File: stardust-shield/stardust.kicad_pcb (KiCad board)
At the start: 2 copper layers, 112.4 x 85.5 mm, 64 parts, among them J1 BEXUS 28V, J2 Pololu J8557, J3 Pololu J8557, J4 Pololu J9251, J5 Pololu J9251 Servo, J6 DS3231M, J7 VMA430, J7'1 VMA430, SW1 SW_Push, SW2 SW_Push, U1 INA181, U2 INA181, U3 INA181, U4 INA181, U5 DS18B20, U6 DS18B20, U8 DHT22, U9 SSCDRNN015PASA5

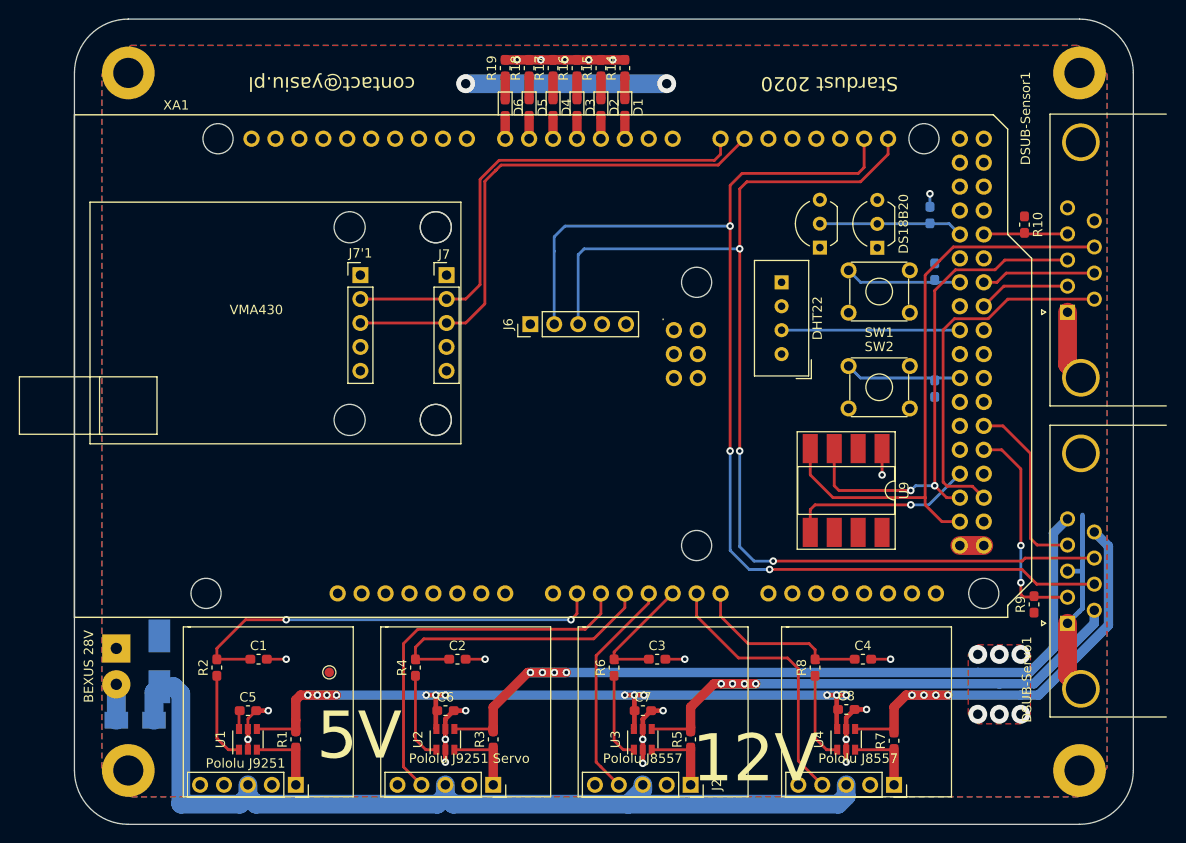
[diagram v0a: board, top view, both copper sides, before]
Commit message: change everything
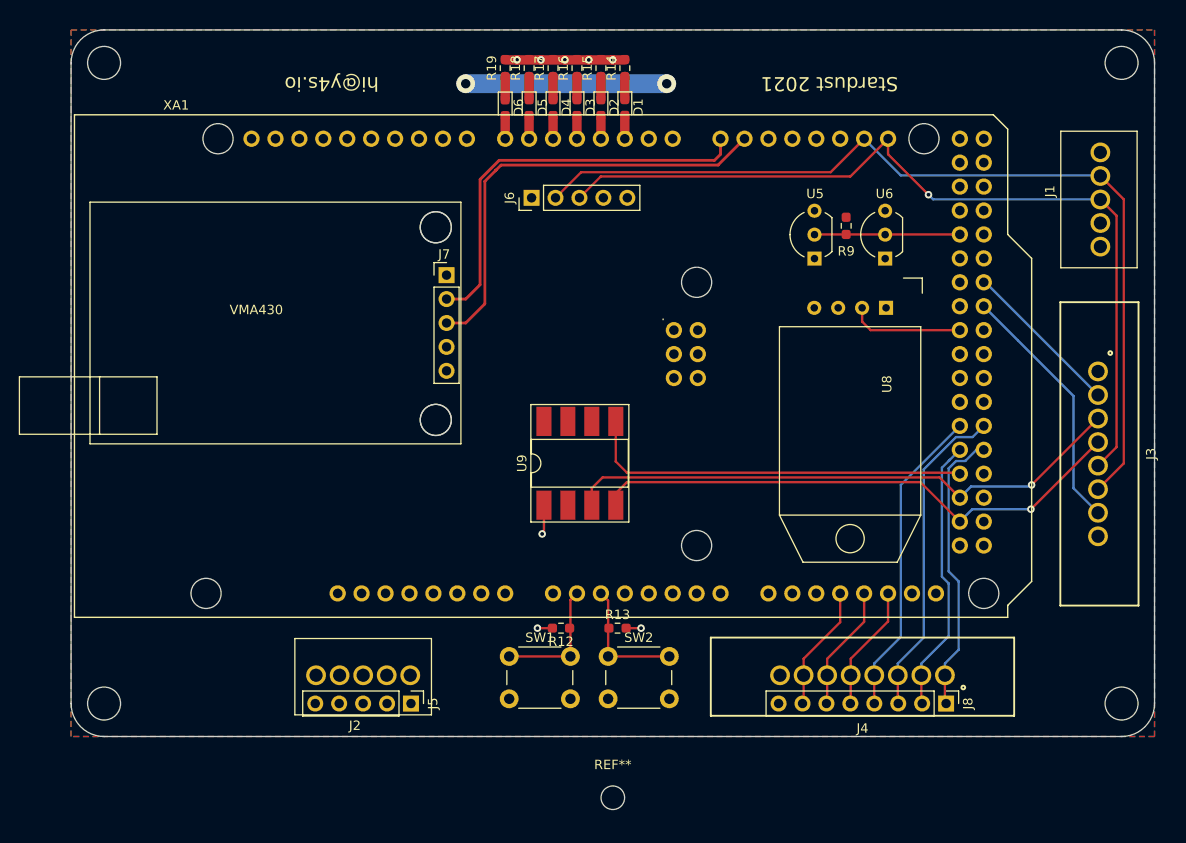
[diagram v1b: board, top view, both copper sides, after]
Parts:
- removed C1, C2, C3, C4: 1uF, Capacitor_SMD:C_0603_1608Metric_Pad1.05x0.95mm_HandSolder
- removed C5, C6, C7, C8: 100uF, Capacitor_SMD:C_0603_1608Metric_Pad1.05x0.95mm_HandSolder
- removed D7: D_TVS, Diode_SMD:D_SMB_Handsoldering
- removed D8: D_Schottky, Diode_SMD:D_SMA
- removed DSUB-Sensor1, DSUB-Servo1: DB9_Male_MountingHoles, Connector_Dsub:DSUB-9_Male_Horizontal_P2.77x2.84mm_EdgePinOffset7.70mm_Housed_MountingHolesOffset9.12mm
- removed J7'1: VMA430, Connector_PinHeader_2.54mm:PinHeader_1x05_P2.54mm_Vertical
- removed R1, R3, R5, R7: 200m, Resistor_SMD:R_0603_1608Metric_Pad1.05x0.95mm_HandSolder
- removed R10, R11: 4.7k, Resistor_SMD:R_0603_1608Metric_Pad1.05x0.95mm_HandSolder
- removed R2, R4, R6, R8: 16k, Resistor_SMD:R_0603_1608Metric_Pad1.05x0.95mm_HandSolder
- removed the REF** at (146.8, 141.6)
- removed the REF** at (73.4, 139.2)
- removed the REF** at (144.5, 140.5)
- removed the REF** at (142.2, 139.2)
- removed the REF** at (153.0, 149.6)
- removed the REF** at (153.0, 75.6)
- removed the REF** at (52.1, 149.6)
- removed the REF** at (52.1, 75.6)
- removed U1, U2, U3, U4: INA181, Package_TO_SOT_SMD:SOT-23-6
- added J8: Power PCB Goldpin, Connector_PinHeader_2.54mm:PinHeader_1x08_P2.54mm_Vertical, F.Cu at (138.9, 142.5)
- added REF**: MountingHole_3.5mm, MountingHole:MountingHole_3.5mm, F.Cu at (49.5, 142.5)
- added REF**: MountingHole_3.5mm, MountingHole:MountingHole_3.5mm, F.Cu at (157.5, 142.5)
- added REF**: MountingHole_3.5mm, MountingHole:MountingHole_3.5mm, F.Cu at (157.5, 74.5)
- added REF**: MountingHole_3.5mm, MountingHole:MountingHole_3.5mm, F.Cu at (49.5, 74.5)
- added REF**: MountingHole_2.5mm, MountingHole:MountingHole_2.5mm, F.Cu at (103.5, 152.5)
- J1: value BEXUS 28V -> Experiment PCB; footprint Connector_Wire:SolderWirePad_1x02_P3.81mm_Drill1.2mm -> Stardust:691382000005
- J2: value Pololu J8557 -> Power PCB; footprint Connector_PinSocket_2.54mm:PinSocket_1x05_P2.54mm_Vertical -> Stardust:691382000005
- J3: value Pololu J8557 -> Sensor PCB; footprint Connector_PinSocket_2.54mm:PinSocket_1x05_P2.54mm_Vertical -> Stardust:691382030008
- J4: value Pololu J9251 -> Power PCB; footprint Connector_PinSocket_2.54mm:PinSocket_1x05_P2.54mm_Vertical -> Stardust:691382030008
- J5: value Pololu J9251 Servo -> Power PCB Goldpin; footprint Connector_PinSocket_2.54mm:PinSocket_1x05_P2.54mm_Vertical -> Connector_PinHeader_2.54mm:PinHeader_1x05_P2.54mm_Vertical
- R12, R13: footprint Resistor_SMD:R_0603_1608Metric_Pad1.05x0.95mm_HandSolder -> Resistor_SMD:R_0603_1608Metric_Pad0.98x0.95mm_HandSolder; moved to F.Cu
- R14, R15, R16, R17, R18, R19, R9: footprint Resistor_SMD:R_0603_1608Metric_Pad1.05x0.95mm_HandSolder -> Resistor_SMD:R_0603_1608Metric_Pad0.98x0.95mm_HandSolder
- SW1, SW2: footprint Button_Switch_THT:SW_TH_Tactile_Omron_B3F-10xx -> Button_Switch_THT:SW_PUSH_6mm
- U8: footprint Sensor:Aosong_DHT11_5.5x12.0_P2.54mm -> Stardust:DHT22_15.0x25.0_P2.54mm_Horizontal
- moved J1 114.8 mm to (155.2, 89.0), turned to 90 degrees
- moved J4 61.3 mm to (130.0, 139.5), turned to 180 degrees
- moved R12 54.8 mm to (98.0, 134.5), turned to 180 degrees
- moved SW1 54.6 mm to (92.5, 137.5)
- moved R9 44.9 mm to (128.3, 91.8), turned to -90 degrees
- moved R13 42.2 mm to (104.0, 134.5), turned to 0 degrees
- moved J3 41.3 mm to (155.0, 116.0)
- moved SW2 40.0 mm to (103.0, 137.5)
- moved J2 36.7 mm to (77.0, 139.5), turned to 180 degrees
- moved U9 28.4 mm to (100.0, 117.0), turned to 90 degrees
- moved J6 13.4 mm to (94.9, 88.8)
- moved J5 12.3 mm to (82.1, 142.5)
- moved U8 12.1 mm to (132.5, 100.5), turned to -90 degrees
- moved U6 7.03 mm to (132.4, 95.3)
- moved U5 6.76 mm to (124.9, 95.3)
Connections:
- J1 pad 1: GND -> +5V
- J1 pad 2: Net-(D8-Pad2) -> (no net)
- J2 pad 1: Net-(J2-Pad1) -> +5V
- J2 pad 2: GND -> +5V
- J2 pad 3: +28V -> +5V
- J2 pad 4: DC-Pump-1 -> GND
- J2 pad 5: Net-(J2-Pad5) -> GND
- J3 pad 1: Net-(J3-Pad1) -> +5V
- J3 pad 2: GND -> SPI-SS-Pressure-1
- J3 pad 3: +28V -> SPI-MISO
- J3 pad 4: DC-Pump-2 -> SPI-CLK
- J3 pad 5: Net-(J3-Pad5) -> I2C-SCL
- J4 pad 1: Net-(J4-Pad1) -> Servo-GPIO
- J4 pad 2: GND -> Heating-PWM
- J4 pad 3: +28V -> Pump-1-PWM
- J4 pad 4: Net-(J4-Pad4) -> Pump-2-PWM
- J4 pad 5: Net-(J4-Pad5) -> INA1
- J5 pad 1: Net-(J5-Pad1) -> +5V
- J5 pad 2: GND -> +5V
- J5 pad 3: +28V -> +5V
- J5 pad 4: DC-Servo -> GND
- J5 pad 5: Net-(J5-Pad5) -> GND
- J6 pad 4: Net-(J6-Pad4) -> (no net)
- J7 pad 1: Net-(J7-Pad1) -> (no net)
- R9 pad 2: 1Wire-1 -> 1Wire
- U5 pad 2: 1Wire-3 -> 1Wire
- U6 pad 2: 1Wire-3 -> 1Wire
- U8 pad 3: Net-(U8-Pad3) -> (no net)
- XA1 pad 3V3: Net-(XA1-Pad3V3) -> (no net)
- XA1 pad 5V1: Net-(XA1-Pad5V1) -> (no net)
- XA1 pad 5V2: Net-(XA1-Pad5V2) -> (no net)
- XA1 pad 5V3: Net-(XA1-Pad5V3) -> (no net)
- XA1 pad 5V4: Net-(XA1-Pad5V4) -> (no net)
- XA1 pad A0: Net-(XA1-PadA0) -> (no net)
- XA1 pad A1: INA1 -> Button-1
- XA1 pad A10: Net-(XA1-PadA10) -> (no net)
- XA1 pad A11: Net-(XA1-PadA11) -> INA3
- XA1 pad A12: Net-(XA1-PadA12) -> INA2
- XA1 pad A13: Net-(XA1-PadA13) -> INA1
- XA1 pad A14: Net-(XA1-PadA14) -> (no net)
- XA1 pad A15: Net-(XA1-PadA15) -> (no net)
- XA1 pad A2: DC-Servo -> Button-2
- XA1 pad A3: INA2 -> (no net)
- XA1 pad A4: DC-Pump-1 -> (no net)
- XA1 pad A5: INA3 -> (no net)
- XA1 pad A6: DC-Pump-2 -> (no net)
- XA1 pad A7: INA4 -> (no net)
- XA1 pad A8: Net-(XA1-PadA8) -> (no net)
- XA1 pad A9: Net-(XA1-PadA9) -> (no net)
- XA1 pad AREF: Net-(XA1-PadAREF) -> (no net)
- XA1 pad D0: Net-(XA1-PadD0) -> (no net)
- XA1 pad D1: Net-(XA1-PadD1) -> (no net)
- XA1 pad D10: Net-(XA1-PadD10) -> (no net)
- XA1 pad D11: Net-(XA1-PadD11) -> (no net)
- XA1 pad D12: Net-(XA1-PadD12) -> (no net)
- XA1 pad D13: Net-(XA1-PadD13) -> (no net)
- XA1 pad D16: TX2 -> (no net)
- XA1 pad D17: RX2 -> (no net)
- XA1 pad D18: TX1 -> (no net)
- XA1 pad D19: RX1 -> (no net)
- XA1 pad D22: Net-(XA1-PadD22) -> (no net)
- XA1 pad D23: Net-(XA1-PadD23) -> (no net)
- XA1 pad D24: Net-(XA1-PadD24) -> (no net)
- XA1 pad D25: Net-(XA1-PadD25) -> (no net)
- XA1 pad D26: Net-(XA1-PadD26) -> (no net)
- XA1 pad D27: Net-(XA1-PadD27) -> (no net)
- XA1 pad D28: 1Wire-3 -> 1Wire
- XA1 pad D29: 1Wire-2 -> (no net)
- XA1 pad D30: Net-(XA1-PadD30) -> (no net)
- XA1 pad D31: Net-(XA1-PadD31) -> (no net)
- XA1 pad D32: Button-1 -> (no net)
- XA1 pad D34: Net-(XA1-PadD34) -> (no net)
- XA1 pad D37: Net-(XA1-PadD37) -> (no net)
- XA1 pad D38: Net-(XA1-PadD38) -> (no net)
- XA1 pad D39: Net-(XA1-PadD39) -> (no net)
- XA1 pad D40: Button-2 -> (no net)
- XA1 pad D41: Net-(XA1-PadD41) -> (no net)
- XA1 pad D42: Net-(XA1-PadD42) -> (no net)
- XA1 pad D43: Net-(XA1-PadD43) -> (no net)
- XA1 pad D44: Net-(XA1-PadD44) -> Pump-2-PWM
- XA1 pad D45: DHT22-1 -> Pump-1-PWM
- XA1 pad D46: Net-(XA1-PadD46) -> Heating-PWM
- XA1 pad D47: 1Wire-1 -> Servo-GPIO
- XA1 pad D49: Net-(XA1-PadD49) -> (no net)
- XA1 pad D51: SPI-MOSI -> (no net)
- XA1 pad D53: Net-(XA1-PadD53) -> (no net)
- XA1 pad D8: Net-(XA1-PadD8) -> (no net)
- XA1 pad D9: Net-(XA1-PadD9) -> (no net)
- XA1 pad GND4: Net-(XA1-PadGND4) -> (no net)
- XA1 pad IORF: Net-(XA1-PadIORF) -> (no net)
- XA1 pad MISO: Net-(XA1-PadMISO) -> (no net)
- XA1 pad MOSI: Net-(XA1-PadMOSI) -> (no net)
- XA1 pad RST1: Net-(XA1-PadRST1) -> (no net)
- XA1 pad RST2: Net-(XA1-PadRST2) -> (no net)
- XA1 pad SCK: Net-(XA1-PadSCK) -> (no net)
- XA1 pad SCL: Net-(XA1-PadSCL) -> (no net)
- XA1 pad SDA: Net-(XA1-PadSDA) -> (no net)
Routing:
- net +28V: track 96.8 -> 0.00 mm
- net +5P: track 91.3 -> 0.00 mm, vias 4 -> 0
- net +5V: track 112.3 -> 21.3 mm, vias 16 -> 2
- net GND: track 82.7 -> 19.0 mm, vias 27 -> 8
- net +12V: track 62.2 -> 0.00 mm, vias 4 -> 0
- net +12P: track 51.5 -> 0.00 mm, vias 4 -> 0
- net DC-Servo: track 40.2 -> 0.00 mm
- net SPI-MOSI: track 38.9 -> 0.00 mm
- net Pump-1-PWM: track 0.00 -> 35.0 mm
- net Pump-2-PWM: track 0.00 -> 33.9 mm
- net INA1: track 46.8 -> 14.1 mm, vias 2 -> 0
- net Servo-GPIO: track 0.00 -> 31.3 mm
- net Heating-PWM: track 0.00 -> 30.1 mm
- net DC-Pump-2: track 28.9 -> 0.00 mm
- net I2C-SCL: track 120.1 -> 91.3 mm, vias 3 -> 1
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- removed copper zone on F.Cu, net GND
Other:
- board size 112.4 x 85.5 mm -> 115 x 75 mm
- net class Default removed
- board text added: "Stardust 2021"
- board text added: "hi@y4s.io"
- board text removed: "12V"
- board text removed: "5V"
- board text removed: "Stardust 2020"
- board text removed: "contact@yasiu.pl"
